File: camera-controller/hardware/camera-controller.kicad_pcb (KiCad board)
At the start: 4 copper layers, 50 x 50 mm, 76 parts, among them J1 USB_C_Receptacle_USB2.0_14P, J2 Conn_Coaxial, J3 Conn_01x04, J4 Conn_01x08, J5 Micro_SD_Card_Det1, J6 Conn_01x02, U1 STM32H523RCTx, U2 LR2021, U3 MIC5504-3.3YM5, Y1 32.768MHz, Y2 24MHz, Y3 32MHz 10pF

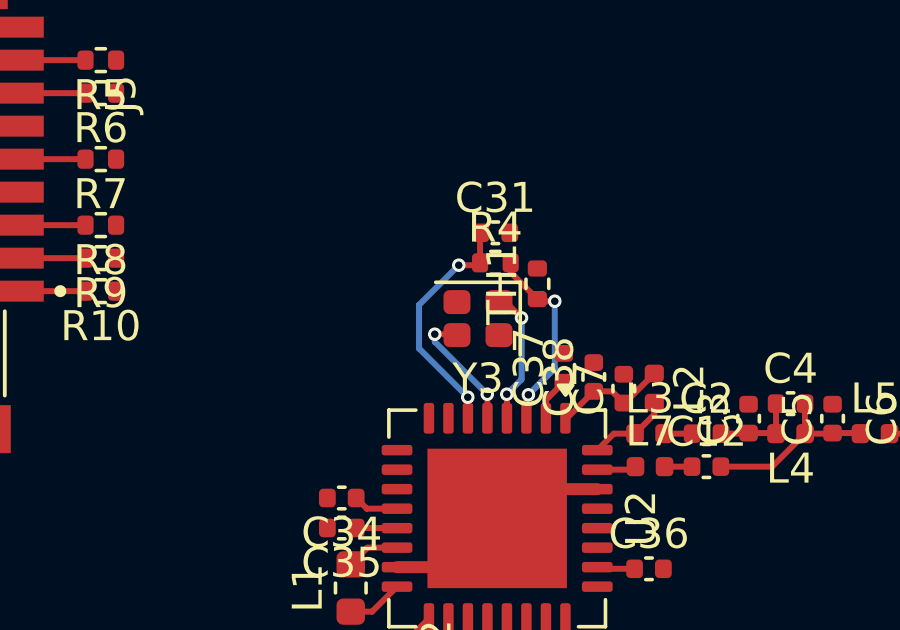
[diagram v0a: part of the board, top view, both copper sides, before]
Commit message: first draft of transceiver pcb
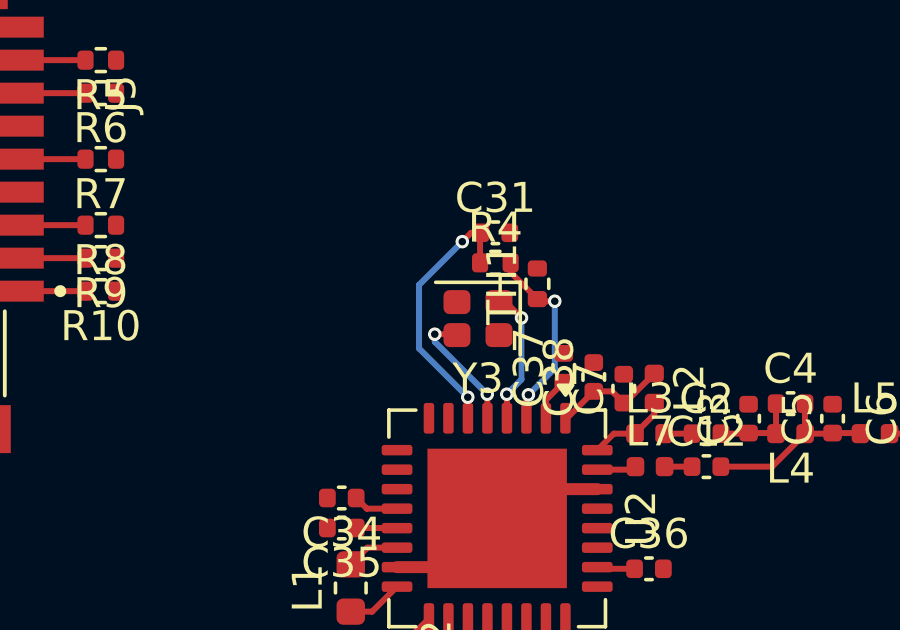
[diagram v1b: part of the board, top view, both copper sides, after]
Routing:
- net /VNTC: track 8.08 -> 9.03 mm
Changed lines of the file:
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@@
+	)
+	(segment
+		(start 137.8825 88.98)
+		(end 137.915 88.98)
+		(width 0.2)
+		(layer "F.Cu")
+		(net "/VR_PA")
+	)
+	(segment
+		(start 135.9375 89.4875)
+		(end 135.985 89.4875)
+		(width 0.2)
+		(layer "F.Cu")
+		(net "/VR_PA")
+	)
+	(segment
+		(start 136.8825 88.59)
+		(end 137.4925 88.59)
+		(width 0.2)
+		(layer "F.Cu")
+		(net "/VR_PA")
+	)
+	(segment
+		(start 135.985 89.4875)
+		(end 136.8825 88.59)
+		(width 0.2)
+		(layer "F.Cu")
+		(net "/VR_PA")
+	)
+	(segment
+		(start 137.915 88.98)
+		(end 138.9 87.995)
+		(width 0.2)
+		(layer "F.Cu")
+		(net "/VR_PA")
+	)
+	(segment
+		(start 137.4925 88.59)
+		(end 137.8825 88.98)
+		(width 0.2)
+		(layer "F.Cu")
+		(net "/VR_PA")
 	)
 	(segment
@@
 		(layer "F.Cu")
 		(net "/VDCD")
-	)
-	(segment
-		(start 137.8825 88.98)
-		(end 137.915 88.98)
-		(width 0.2)
-		(layer "F.Cu")
-		(net "/VR_PA")
-	)
-	(segment
-		(start 135.9375 89.4875)
-		(end 135.985 89.4875)
-		(width 0.2)
-		(layer "F.Cu")
-		(net "/VR_PA")
-	)
-	(segment
-		(start 136.8825 88.59)
-		(end 137.4925 88.59)
-		(width 0.2)
-		(layer "F.Cu")
-		(net "/VR_PA")
-	)
-	(segment
-		(start 135.985 89.4875)
-		(end 136.8825 88.59)
-		(width 0.2)
-		(layer "F.Cu")
-		(net "/VR_PA")
-	)
-	(segment
-		(start 137.915 88.98)
-		(end 138.9 87.995)
-		(width 0.2)
-		(layer "F.Cu")
-		(net "/VR_PA")
-	)
-	(segment
-		(start 137.4925 88.59)
-		(end 137.8825 88.98)
-		(width 0.2)
-		(layer "F.Cu")
-		(net "/VR_PA")
 	)
 	(segment
@@
 	)
 	(segment
+		(start 132.795 83.305)
+		(end 132.5 83.6)
+		(width 0.2)
+		(layer "F.Cu")
+		(net "/VNTC")
+	)
+	(segment
 		(start 133.0125 84.385)
 		(end 133.0925 84.305)
@@
 	)
 	(segment
+		(start 133.0925 84.305)
+		(end 133.0925 83.335)
+		(width 0.2)
+		(layer "F.Cu")
+		(net "/VNTC")
+	)
+	(segment
 		(start 133.0925 83.335)
 		(end 133.1225 83.305)
@@
 	)
 	(segment
-		(start 132.3825 84.385)
-		(end 133.0125 84.385)
-		(width 0.2)
-		(layer "F.Cu")
-		(net "/VNTC")
-	)
-	(segment
-		(start 133.0925 84.305)
-		(end 133.0925 83.335)
+		(start 133.1225 83.305)
+		(end 132.795 83.305)
 		(width 0.2)
 		(layer "F.Cu")
@@
 	)
 	(via
-		(at 132.3825 84.385)
+		(at 132.5 83.6)
 		(size 0.45)
 		(drill 0.25)
@@
 	)
 	(segment
-		(start 131.0575 85.71)
-		(end 132.3825 84.385)
+		(start 132.5 83.6)
+		(end 131.0575 85.0425)
 		(width 0.2)
 		(layer "B.Cu")
@@
 	)
 	(segment
+		(start 131.0575 85.0425)
+		(end 131.0575 87.16)
+		(width 0.2)
+		(layer "B.Cu")
+		(net "/VNTC")
+	)
+	(segment
 		(start 131.0575 87.16)
-		(end 131.0575 85.71)
-		(width 0.2)
-		(layer "B.Cu")
-		(net "/VNTC")
-	)
-	(segment
-		(start 132.6825 88.785)
-		(end 131.0575 87.16)
+		(end 132.6825 88.785)
 		(width 0.2)
 		(layer "B.Cu")
@@
 			"1041f301-0349-46e1-8822-e52b4c8b3ef3" "12806317-d077-4186-afc8-4ff6c8b48ca6"
 			"1358a051-eabb-4d72-8740-a3e8340d7430" "14c4fe99-effd-4213-b37c-9940db8c8617"
-			"1bc62bba-f5a6-4853-8b79-c390b3c4d4ec" "22a04720-38bb-4a67-ac98-641396f7d127"
-			"22eb65f4-8c5d-4586-a4b8-ceda9d763b47" "232033eb-20f1-45d0-afbe-8b199121b99f"
+			"16ea95fa-2117-4c31-b320-c81fa461d456" "1bc62bba-f5a6-4853-8b79-c390b3c4d4ec"
+			"22a04720-38bb-4a67-ac98-641396f7d127" "22eb65f4-8c5d-4586-a4b8-ceda9d763b47"
 			"25ba02d5-fe6b-491c-a444-6947921c7fa2" "294f298a-5d62-4bb4-92fc-3cd66b71c9f3"
 			"297e477f-3bd5-466f-97cc-183f80c5a877" "29bd2dab-4127-43d0-8c59-eb513871ad1f"
@@
 			"3c567c16-5b1a-4103-81fa-bbbf8e89759e" "3db08dd0-9d63-4ba8-9f47-7a111a2e8c16"
 			"3efdddb5-215b-4429-a065-ae92ea39b3f6" "3f8e9e50-f241-46df-8971-e3739bbed58e"
-			"4a98f093-3556-46d0-ac74-e7f70d9f5ed7" "4ad88457-1c89-4308-9773-7be579d44e77"
-			"4b459bfa-e7bc-4b6c-a935-ecee057ecc3f" "4cab0f25-4cdd-44b1-b5d6-e5e464ac5cf2"
-			"4dde2c58-0db9-4dc6-9f62-d341adf25ec6" "5093e0a3-720a-424e-a623-362573196668"
-			"53934e35-9437-4c15-ae4b-0d2993678153" "53a3d976-f4e8-4ba2-bc08-6eafea4ac1b6"
-			"53a878ac-959b-45c6-b73e-98e1f2b09d01" "5407e300-0a74-4397-8c8b-c6f9cd2c627a"
-			"54b8e979-e094-4e20-8895-67b28e4b60d9" "55071383-3d0b-42b2-b6ea-09fe577c875e"
-			"568bfd12-2cd2-43ba-837a-8520e3d8815b" "5e81f525-636d-46cd-bfc2-b39449f61016"
+			"41a4a1db-37e9-47e3-bd20-668b57c9d571" "4a98f093-3556-46d0-ac74-e7f70d9f5ed7"
+			"4ad88457-1c89-4308-9773-7be579d44e77" "4b459bfa-e7bc-4b6c-a935-ecee057ecc3f"
+			"4cab0f25-4cdd-44b1-b5d6-e5e464ac5cf2" "4dde2c58-0db9-4dc6-9f62-d341adf25ec6"
+			"5093e0a3-720a-424e-a623-362573196668" "53934e35-9437-4c15-ae4b-0d2993678153"
+			"53a3d976-f4e8-4ba2-bc08-6eafea4ac1b6" "53a878ac-959b-45c6-b73e-98e1f2b09d01"
+			"5407e300-0a74-4397-8c8b-c6f9cd2c627a" "54b8e979-e094-4e20-8895-67b28e4b60d9"
+			"55071383-3d0b-42b2-b6ea-09fe577c875e" "568bfd12-2cd2-43ba-837a-8520e3d8815b"
 			"5f2cc1a4-7456-4aed-8d9e-5917b5e84710" "6182e8bb-4aff-437f-a52e-73305ee6edba"
-			"635f17a9-e630-4d9d-8210-70e7b36fff07" "63c20438-46f6-4ee7-911a-c58d40576bf5"
+			"62fc68d4-692f-437d-9fc9-3114675058b1" "635f17a9-e630-4d9d-8210-70e7b36fff07"
 			"649eaf3d-14d1-4637-bd7a-8235cbd74dd0" "67316d8f-cc4c-4789-b70e-fcd437be1d97"
 			"695e444d-a78e-4130-94c7-af668493d3ea" "6ac16a02-b0d6-4459-bc49-bbcd1f473ad5"
 			"6f00eed7-eb88-4b59-862a-3584900a57c5" "720c3742-8d0d-4a1a-84fd-ceab40c7a67b"
-			"72d330eb-cf0a-423a-af3e-0f59053a2d27" "75741f89-70f7-48fc-9717-0e1a88b932ea"
-			"7674c199-ece3-4afe-8abe-5e29dfa1b6c8" "76a4131d-5475-43ff-8108-0c747d10cfba"
-			"7e145a3e-3f4d-41e9-b5c6-59e226b69e31" "849efa61-3214-4e4a-af83-0731b5feaaf1"
-			"85945e1c-906f-4803-88b2-e16dfa261972" "8a0f1625-f3a6-419f-a61d-bdda690c43e8"
-			"8d874a64-ccb8-438f-92f7-6ada4d00b5d6" "8f86705f-1f0d-4cf8-8f86-7cc5bea4383c"
-			"90ef851c-f283-4d14-ae3a-faacd81f9eaa" "90f95589-5d6c-458d-b048-59728280ffc3"
-			"91911e61-ecf4-4a3a-a55f-f5137acb9df1" "93b8f4ad-d73d-465a-afc3-d70fe772508d"
-			"9411ef35-6e01-47a7-9445-889dcfd4d362" "9533d95d-7d10-45de-aab2-1e666e29bfc4"
-			"96cbc3c5-6301-40fe-afed-c61fb076f1e6" "97cdcbf2-7e5a-4959-944d-bb05dcb87c5a"
-			"9b83c45e-93b8-4577-bb80-e9d2b3b52471" "9b9628f7-a1d7-499f-a8f7-0582cfc36f20"
-			"a7f143a2-e1f0-4685-b604-fcbac470debd" "aff4eafe-7124-464e-a98c-1847028352bc"
-			"b1bdddd2-c456-4039-90d6-b6281ad746cb" "b2a97659-9143-472e-a058-dcf9368037fd"
+			"72d330eb-cf0a-423a-af3e-0f59053a2d27" "7674c199-ece3-4afe-8abe-5e29dfa1b6c8"
+			"76a4131d-5475-43ff-8108-0c747d10cfba" "7e145a3e-3f4d-41e9-b5c6-59e226b69e31"
+			"849efa61-3214-4e4a-af83-0731b5feaaf1" "85945e1c-906f-4803-88b2-e16dfa261972"
+			"8a0f1625-f3a6-419f-a61d-bdda690c43e8" "8d874a64-ccb8-438f-92f7-6ada4d00b5d6"
+			"8f86705f-1f0d-4cf8-8f86-7cc5bea4383c" "90ef851c-f283-4d14-ae3a-faacd81f9eaa"
+			"90f95589-5d6c-458d-b048-59728280ffc3" "91911e61-ecf4-4a3a-a55f-f5137acb9df1"
+			"93b8f4ad-d73d-465a-afc3-d70fe772508d" "9411ef35-6e01-47a7-9445-889dcfd4d362"
+			"9533d95d-7d10-45de-aab2-1e666e29bfc4" "96cbc3c5-6301-40fe-afed-c61fb076f1e6"
+			"97cdcbf2-7e5a-4959-944d-bb05dcb87c5a" "9b83c45e-93b8-4577-bb80-e9d2b3b52471"
+			"9b9628f7-a1d7-499f-a8f7-0582cfc36f20" "a7f143a2-e1f0-4685-b604-fcbac470debd"
+			"a94a33b1-ec3a-4786-810a-3eeae708a369" "abc65c81-b8fd-445e-ac8e-9e2747afd620"
+			"aff4eafe-7124-464e-a98c-1847028352bc" "b1bdddd2-c456-4039-90d6-b6281ad746cb"
 			"b835949e-edba-4653-8c6a-576bc1b88d6c" "bb30fddc-0220-4993-a194-7e83466d521d"
 			"bcd33461-d973-4b4d-b735-e3e06b90e1d1" "bdb85e52-b1be-45e6-bb12-bc199d1fdd7f"
@@
 			"c5f2284a-7ea0-4470-9b35-ee9dadfd42aa" "c80ebf6f-8e0a-4934-ac7b-74e1ed840b3d"
 			"c8410ad5-1991-4611-bc05-fd26bc2dbf81" "ca0ad787-952d-4f69-9e1e-b1de511cfd63"
-			"cd62c01a-79e3-4cc3-8e91-04355e55cb51" "ce8f2ddd-a142-48f1-8302-e4928810bbbb"
-			"d059787a-41eb-4459-9b92-2bc2f974cbd5" "d2724d46-31c9-461b-b6f8-bc8ed4a375e8"
-			"d3db9992-162a-413c-add7-707a124ae330" "d689d873-4c1c-4f05-821c-25bfc899cac7"
-			"d7723886-3e24-4ac6-b601-714c50871033" "da51e7eb-8af1-46fc-a686-1555ca50d49c"
-			"de00b40c-f0a4-4855-99b1-0134baa2c68a" "ea8869f9-0015-4535-a6bd-c59bbf5a7232"
+			"ce8f2ddd-a142-48f1-8302-e4928810bbbb" "d059787a-41eb-4459-9b92-2bc2f974cbd5"
+			"d2724d46-31c9-461b-b6f8-bc8ed4a375e8" "d3db9992-162a-413c-add7-707a124ae330"
+			"d689d873-4c1c-4f05-821c-25bfc899cac7" "d7723886-3e24-4ac6-b601-714c50871033"
+			"da51e7eb-8af1-46fc-a686-1555ca50d49c" "de00b40c-f0a4-4855-99b1-0134baa2c68a"
+			"dfdfefcf-16e8-44b0-a5d3-4760554c8ce5" "ea8869f9-0015-4535-a6bd-c59bbf5a7232"
 			"ebbd6a3b-182f-47ea-be82-10a87831473f" "ec00e219-6db6-48f9-8c29-6f43fb25f26b"
-			"ec80b570-f99b-4a77-9512-1e8a8d8c6b10" "ee09e8fc-de5e-4cd6-b59c-862bca51a696"
-			"f111fdb8-8d0c-43ce-a812-f9c0d61d8081" "f3fe035a-4c7c-4c7c-b576-b7ed83b3ddcb"
-			"f66bdb33-c91a-4fce-9f2d-7c63be4f6b6f" "f72c7c3a-47da-48b5-adee-efe35439dea7"
-			"f8804ffa-7350-49da-be8d-2334f7638e7e" "f93c4614-8cdd-4a7b-8ce0-35ce11aafb43"
-			"fdcd65bc-2984-43d5-86df-5367c3f8b5ab" "feaef577-9b75-4cfd-a564-bb67bc0ca13f"
+			"ec5d37f8-32bd-43e4-adc1-4cde7720c741" "ec80b570-f99b-4a77-9512-1e8a8d8c6b10"
+			"ee09e8fc-de5e-4cd6-b59c-862bca51a696" "f111fdb8-8d0c-43ce-a812-f9c0d61d8081"
+			"f3fe035a-4c7c-4c7c-b576-b7ed83b3ddcb" "f66bdb33-c91a-4fce-9f2d-7c63be4f6b6f"
+			"f72c7c3a-47da-48b5-adee-efe35439dea7" "f8804ffa-7350-49da-be8d-2334f7638e7e"
+			"f93c4614-8cdd-4a7b-8ce0-35ce11aafb43" "fdcd65bc-2984-43d5-86df-5367c3f8b5ab"
+			"feaef577-9b75-4cfd-a564-bb67bc0ca13f"
 		)
 	)

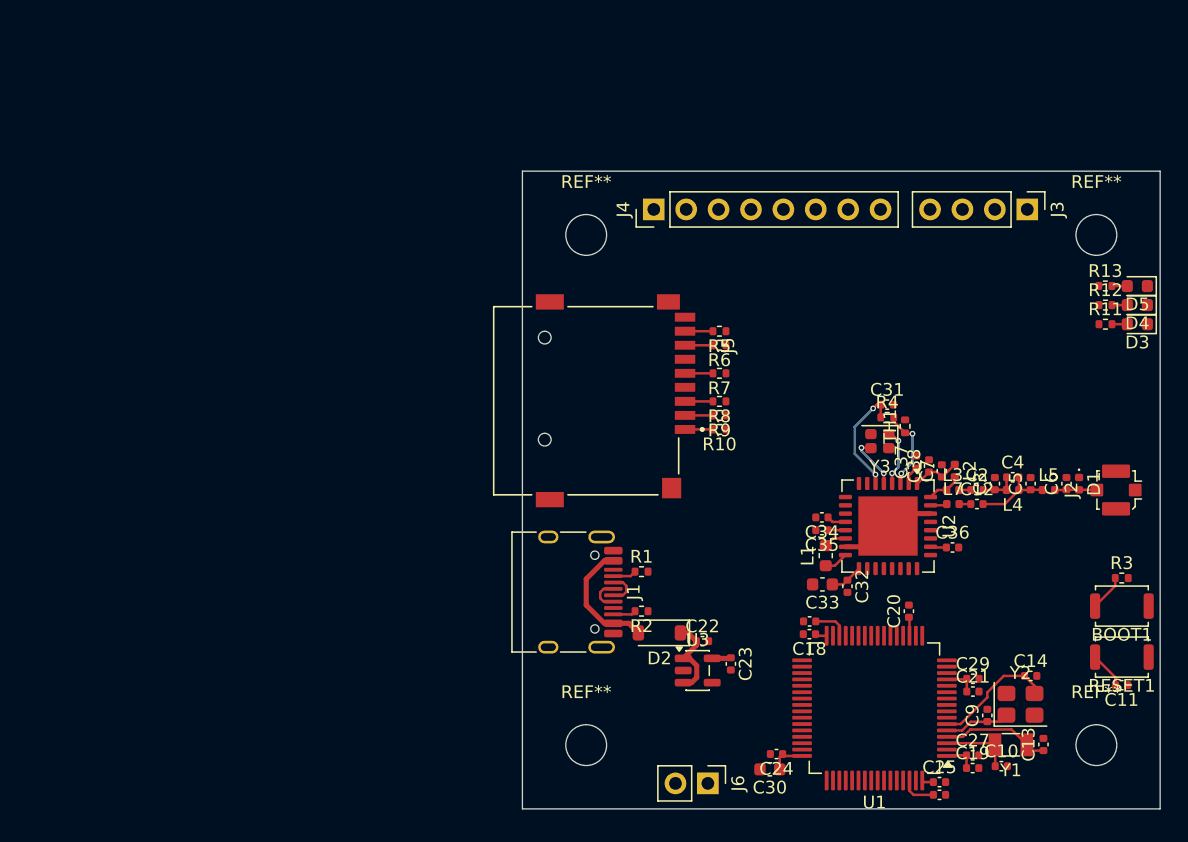
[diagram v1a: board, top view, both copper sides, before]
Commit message: updated board and started frame
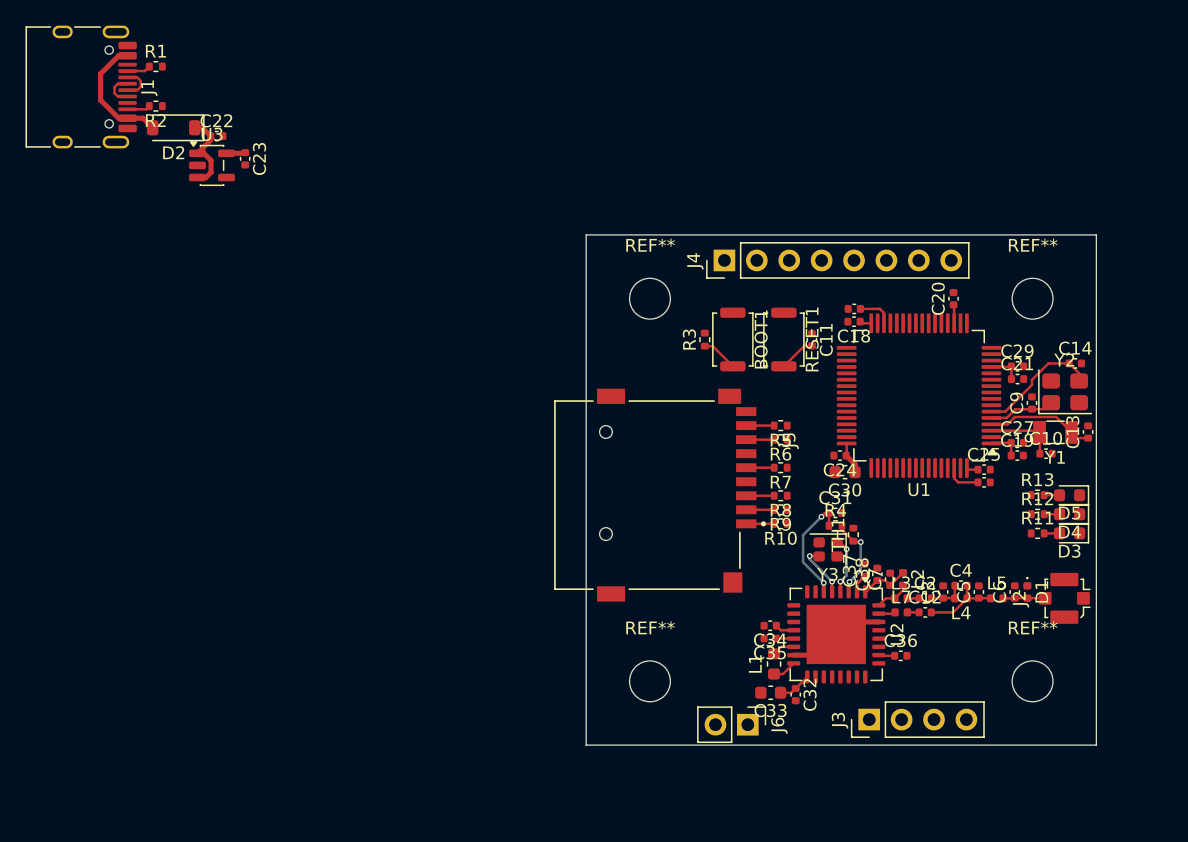
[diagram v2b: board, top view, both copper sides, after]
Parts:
- moved C22 54.9 mm to (81.0, 62.2)
- moved R1 54.9 mm to (76.3, 56.8)
- moved U3 54.9 mm to (80.7, 64.5)
- moved D2 54.9 mm to (77.7, 61.6)
- moved J1 54.9 mm to (70.0, 58.4)
- moved R2 54.9 mm to (76.3, 59.9)
- moved C23 54.9 mm to (83.3, 64.0)
- moved J3 41.9 mm to (132.2, 108.0), turned to 90 degrees
- moved R3 37.7 mm to (119.3, 78.2), turned to 90 degrees
- moved BOOT1 37.0 mm to (121.5, 78.2), turned to -90 degrees
- moved C11 36.4 mm to (127.7, 78.2), turned to -90 degrees
- moved RESET1 36.4 mm to (125.5, 78.2), turned to -90 degrees
- moved C10 24.7 mm to (146.1, 87.2)
- moved C13 24.7 mm to (149.3, 85.5)
- moved C14 24.7 mm to (148.3, 80.1)
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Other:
- board size 50 x 50 mm -> 40 x 40 mm
